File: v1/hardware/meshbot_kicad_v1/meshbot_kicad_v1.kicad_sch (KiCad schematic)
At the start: 20 parts, among them J1 Conn_01x02_Socket, J2 Conn_01x04_Pin, J3 Conn_01x04_Pin, J4 Conn_01x01_Socket, J5 Conn_01x04_Pin, SW1 SW_Push, SW2 SW_Push, SW3 SW_Push, SW4 SW_Push, U1 wio-sx1262, U2 nice_nano_clean, U3 nice_nano_clean, U4 grove_a, U5 grove_a

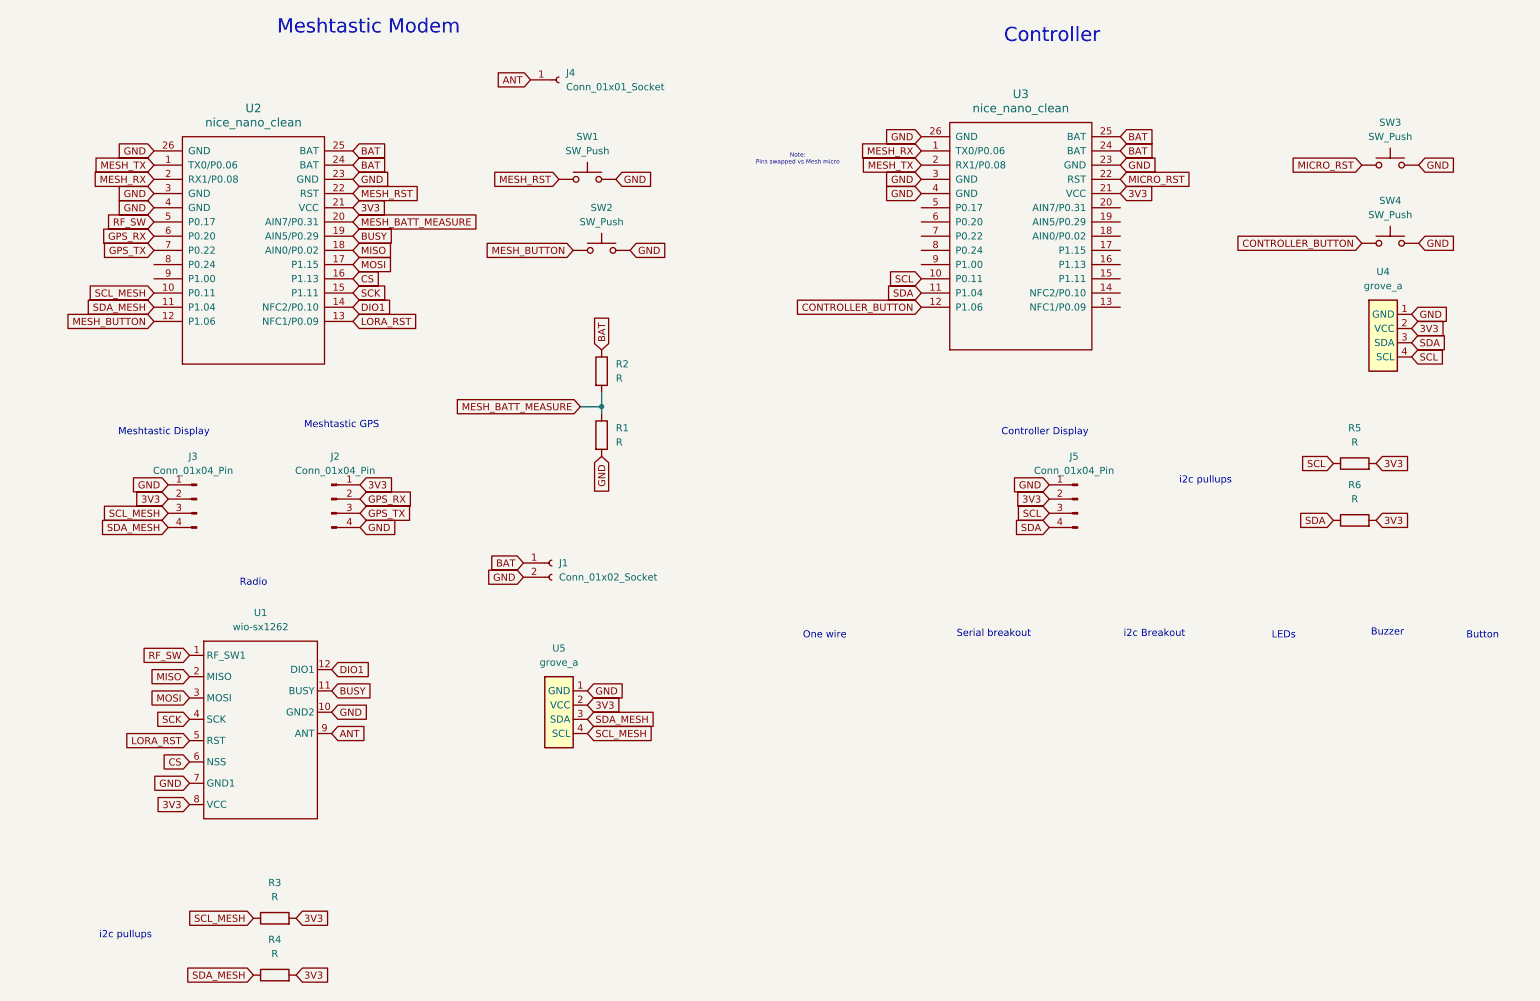
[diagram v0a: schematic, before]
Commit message: update
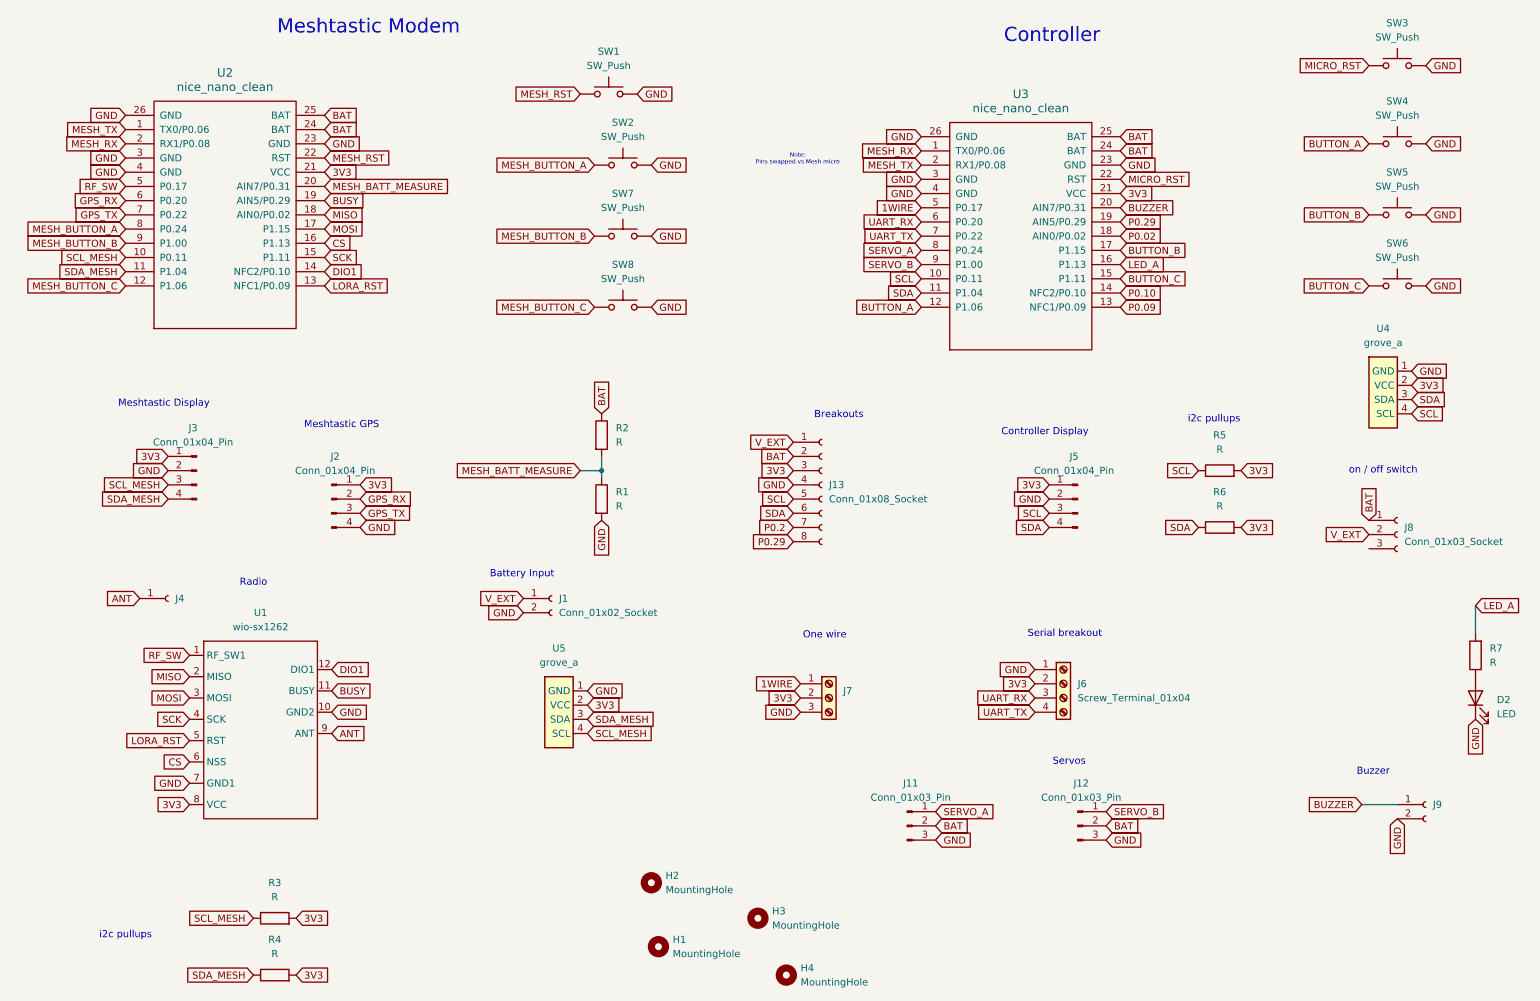
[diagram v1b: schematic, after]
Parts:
- added D2: LED, LED_THT:LED_D5.0mm, symbol Device:LED
- added H1, H2, H3, H4: MountingHole, MountingHole:MountingHole_3.2mm_M3, symbol Mechanical:MountingHole
- added J11, J12: Conn_01x03_Pin, Connector_PinHeader_2.54mm:PinHeader_1x03_P2.54mm_Vertical, symbol Connector:Conn_01x03_Pin
- added J13: Conn_01x08_Socket, Connector_PinSocket_2.54mm:PinSocket_1x08_P2.54mm_Vertical, symbol Connector:Conn_01x08_Socket
- added J6: Screw_Terminal_01x04, TerminalBlock_Phoenix:TerminalBlock_Phoenix_MKDS-1,5-4-5.08_1x04_P5.08mm_Horizontal, symbol Connector:Screw_Terminal_01x04
- added J7: Screw_Terminal_01x03, TerminalBlock_Phoenix:TerminalBlock_Phoenix_MKDS-1,5-3-5.08_1x03_P5.08mm_Horizontal, symbol Connector:Screw_Terminal_01x03
- added J8: Conn_01x03_Socket, footprints:usual_switch, symbol Connector:Conn_01x03_Socket
- added J9: Conn_01x02_Socket, Buzzer_Beeper:Buzzer_12x9.5RM7.6, symbol Connector:Conn_01x02_Socket
- added R7: R, Resistor_THT:R_Axial_DIN0204_L3.6mm_D1.6mm_P1.90mm_Vertical, symbol Device:R
- added SW5, SW6, SW7, SW8: SW_Push, Button_Switch_THT:SW_Tactile_SPST_Angled_PTS645Vx31-2LFS, symbol Switch:SW_Push
- J2: footprint Connector_PinHeader_2.54mm:PinHeader_1x04_P2.54mm_Vertical -> footprints:gps_ublox_blue
- J3, J5: footprint Connector_PinHeader_2.54mm:PinHeader_1x04_P2.54mm_Vertical -> footprints:ssd1306_a
- R3, R4, R5, R6: footprint (none) -> Resistor_THT:R_Axial_DIN0204_L3.6mm_D1.6mm_P1.90mm_Vertical
- SW1, SW2, SW3, SW4: footprint Button_Switch_THT:SW_PUSH_6mm -> Button_Switch_THT:SW_Tactile_SPST_Angled_PTS645Vx31-2LFS
- U4: footprint footprints:grove_rightangle -> footprints:grove_a
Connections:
- net 3V3: now also J3.1 (Pin_1), J5.1 (Pin_1), J13.3 (Pin_3), J6.2 (Pin_2), J7.2 (Pin_2); no longer J3.2 (Pin_2), J5.2 (Pin_2)
- net BAT: now also J11.2 (Pin_2), J12.2 (Pin_2), J13.2 (Pin_2), J8.1 (Pin_1); no longer J1.1 (Pin_1)
- net GND: now also J3.2 (Pin_2), J5.2 (Pin_2), D2.1 (K), J11.3 (Pin_3), J12.3 (Pin_3), J13.4 (Pin_4), J6.1 (Pin_1), J7.3 (Pin_3), J9.2 (Pin_2), SW5.2, SW6.2, SW7.2, SW8.2; no longer J3.1 (Pin_1), J5.1 (Pin_1)
- net SCL: now also J13.5 (Pin_5)
- net SDA: now also J13.6 (Pin_6)
- net MESH_BUTTON_A: now reaches U2.8 (P0.24)
- net MESH_BUTTON_A: now also SW2.1
- net MESH_BUTTON_B: now reaches U2.9 (P1.00)
- net MESH_BUTTON_B: now also SW7.1
- net P0.09: now reaches U3.13 (NFC1/P0.09)
- net P0.10: now reaches U3.14 (NFC2/P0.10)
- net BUTTON_C: now reaches U3.15 (P1.11)
- net BUTTON_C: now also SW6.1
- net LED_A: now reaches U3.16 (P1.13)
- net LED_A: now also R7.2
- net BUTTON_B: now reaches U3.17 (P1.15)
- net BUTTON_B: now also SW5.1
- net P0.02: now reaches U3.18 (AIN0/P0.02)
- net P0.29: now reaches U3.19 (AIN5/P0.29)
- net P0.29: now also J13.8 (Pin_8)
- net BUZZER: now reaches U3.20 (AIN7/P0.31)
- net BUZZER: now also J9.1 (Pin_1)
- net 1WIRE: now reaches U3.5 (P0.17)
- net 1WIRE: now also J7.1 (Pin_1)
- net UART_RX: now reaches U3.6 (P0.20)
- net UART_RX: now also J6.3 (Pin_3)
- net UART_TX: now reaches U3.7 (P0.22)
- net UART_TX: now also J6.4 (Pin_4)
- net SERVO_A: now reaches U3.8 (P0.24)
- net SERVO_A: now also J11.1 (Pin_1)
- net SERVO_B: now reaches U3.9 (P1.00)
- net SERVO_B: now also J12.1 (Pin_1)
- net CONTROLLER_BUTTON renamed BUTTON_A
- net MESH_BUTTON renamed MESH_BUTTON_C
- net MESH_BUTTON_C: now also SW8.1; no longer SW2.1
- new net: D2.2 (A), R7.1
- new net P0.2: J13.7 (Pin_7)
- new net V_EXT: J1.1 (Pin_1), J13.1 (Pin_1), J8.2 (Pin_2)
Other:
- note added: "Battery Input"
- note added: "Breakouts"
- note added: "Servos"
- note added: "on / off switch"
- note removed: "Button"
- note removed: "LEDs"
- note removed: "i2c Breakout"
- moved on the sheet: J1, J3, J4, R1, R2, R5, R6, SW1, SW2, SW3, SW4, U2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

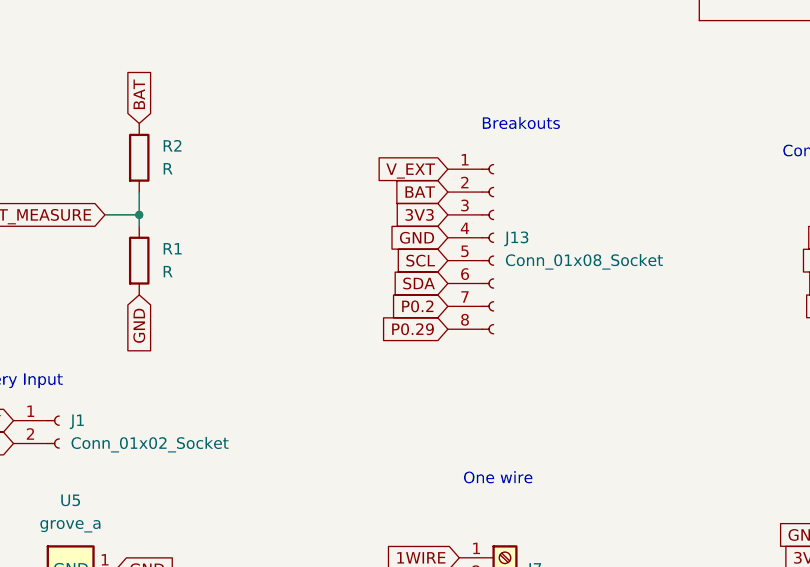
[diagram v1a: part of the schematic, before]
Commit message: update
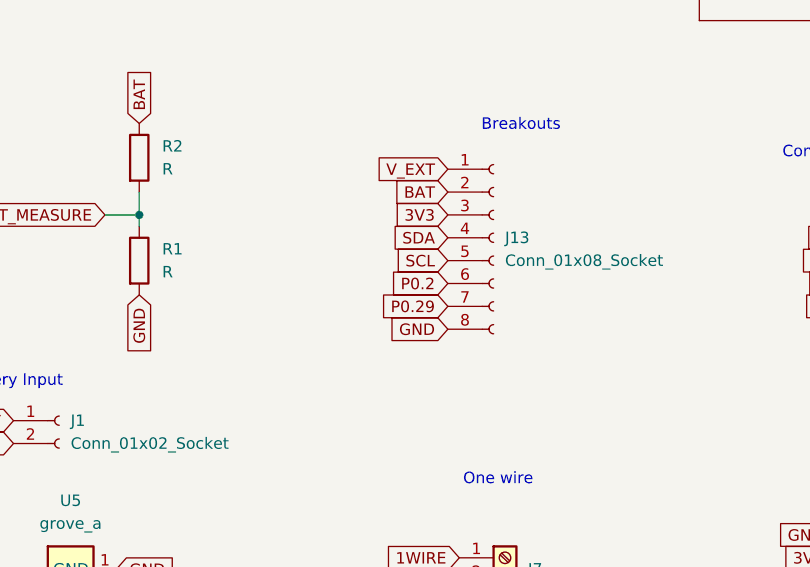
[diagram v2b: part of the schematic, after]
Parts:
- D2: footprint LED_THT:LED_D5.0mm -> LED_THT:LED_D3.0mm
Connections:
- net GND: now also J13.8 (Pin_8); no longer J13.4 (Pin_4)
- net P0.2: now also J13.6 (Pin_6); no longer J13.7 (Pin_7)
- net P0.29: now also J13.7 (Pin_7); no longer J13.8 (Pin_8)
- net SDA: now also J13.4 (Pin_4); no longer J13.6 (Pin_6)

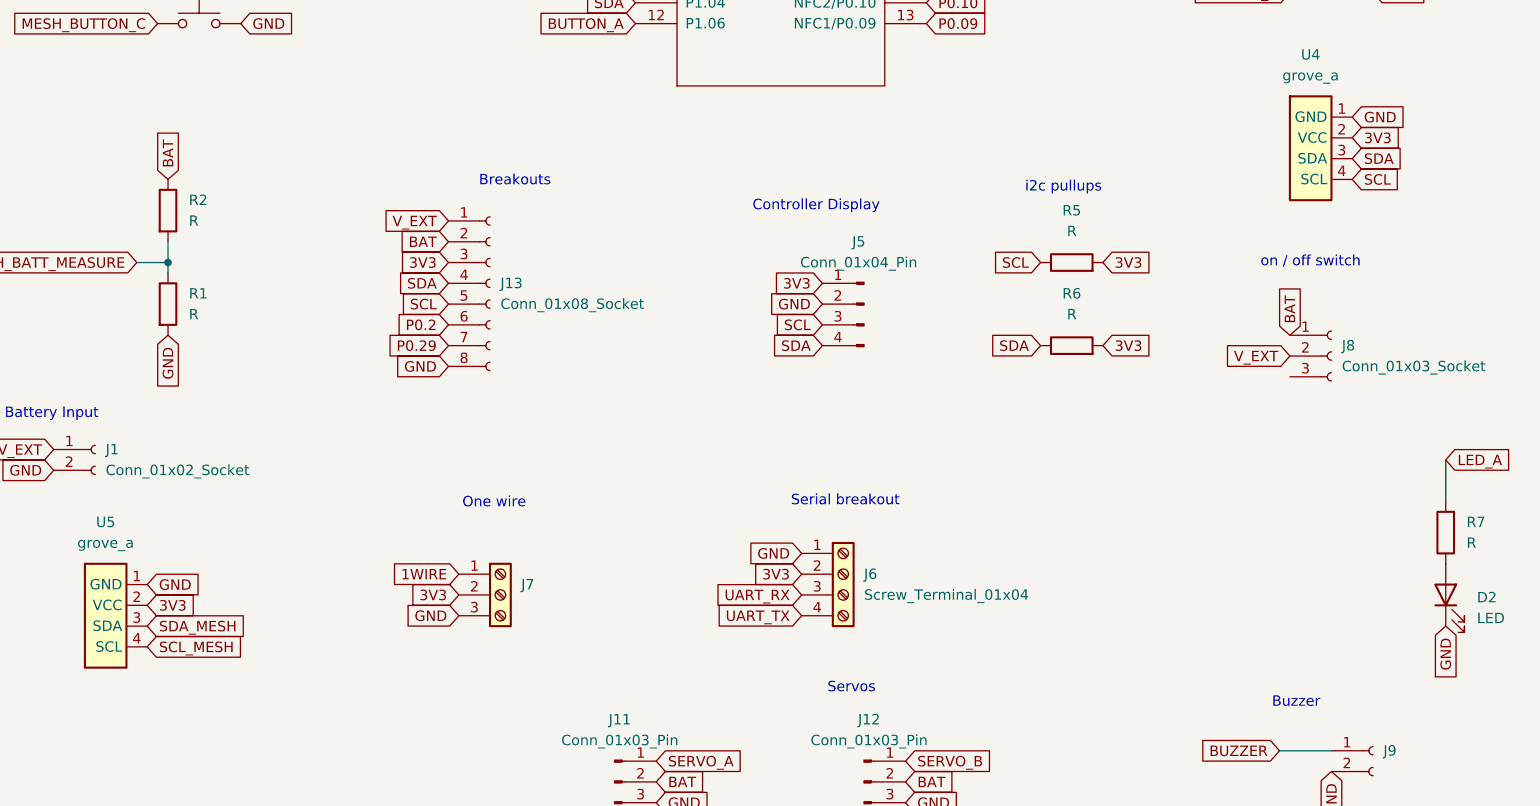
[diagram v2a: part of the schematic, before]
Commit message: update
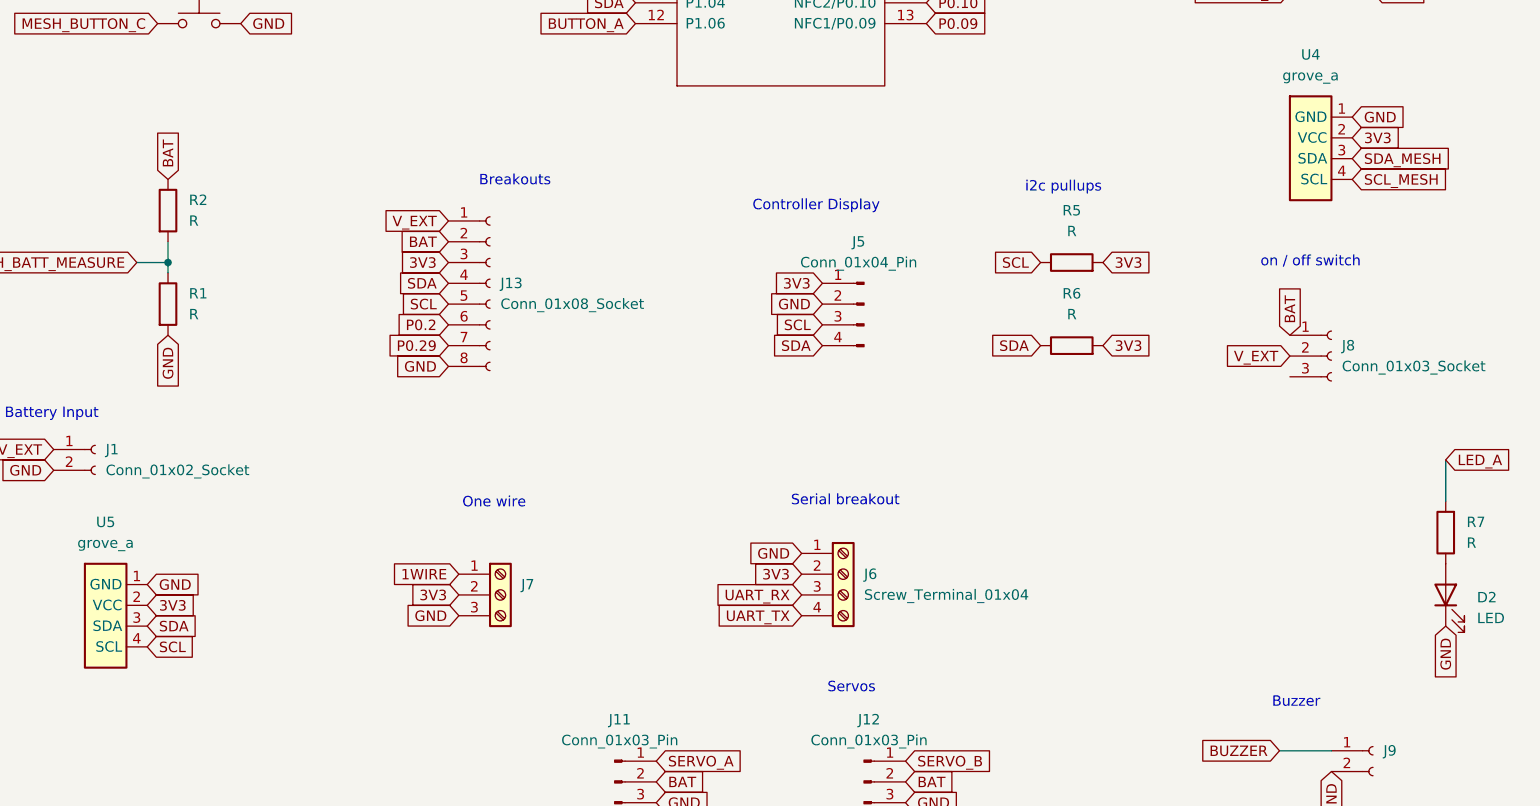
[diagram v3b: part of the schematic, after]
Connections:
- net SCL: now also U5.4 (SCL); no longer U4.4 (SCL)
- net SCL_MESH: now also U4.4 (SCL); no longer U5.4 (SCL)
- net SDA: now also U5.3 (SDA); no longer U4.3 (SDA)
- net SDA_MESH: now also U4.3 (SDA); no longer U5.3 (SDA)
